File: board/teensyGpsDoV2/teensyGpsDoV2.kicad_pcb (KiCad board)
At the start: 2 copper layers, 12 parts, among them J1 Barrel_Jack, J2 NPPN042AFCN-RC, U1 Teensy4.0, U2 LT1086-5.0, U3 DAC8550IxDGK, X1 OSC5A2B02

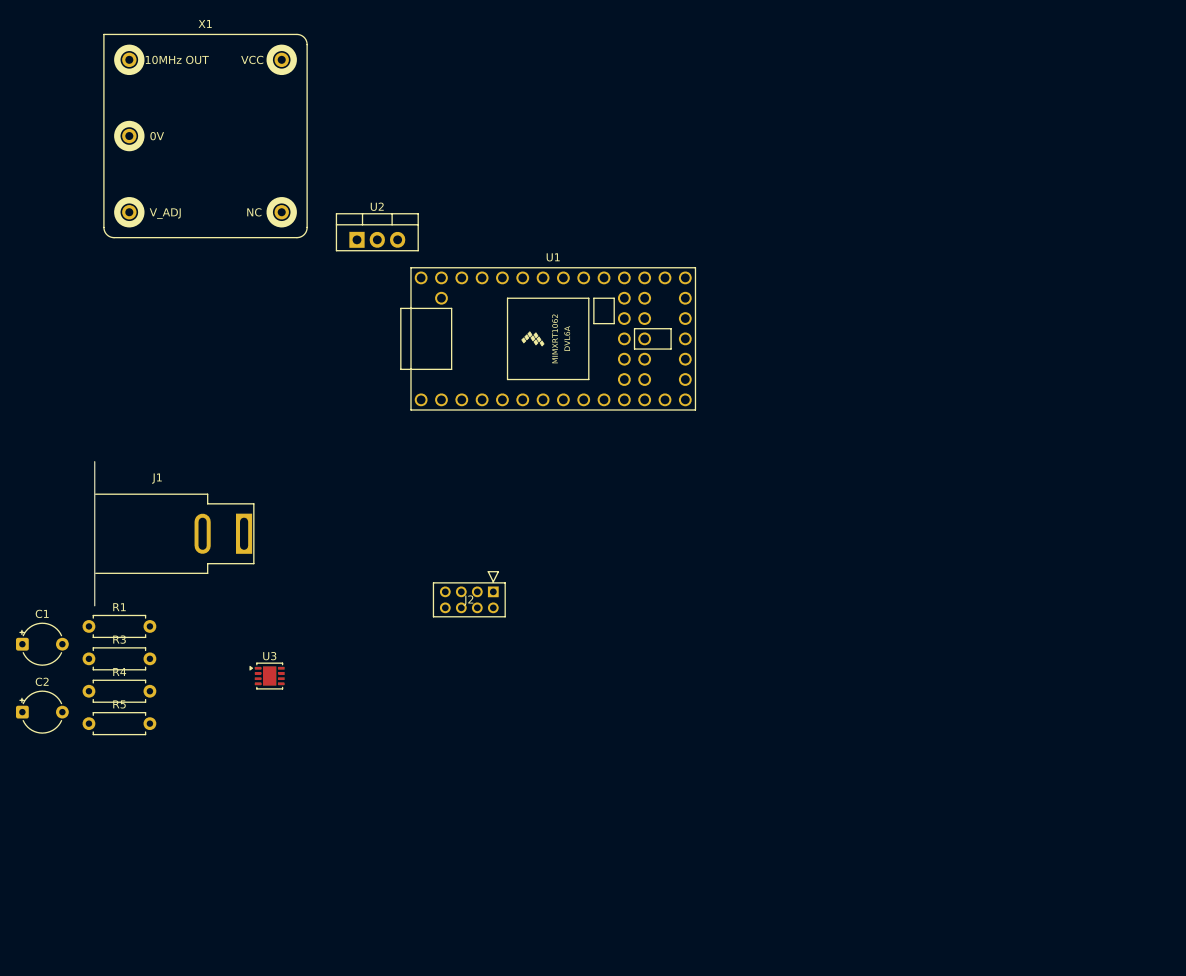
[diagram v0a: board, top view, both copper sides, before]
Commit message: layout wip
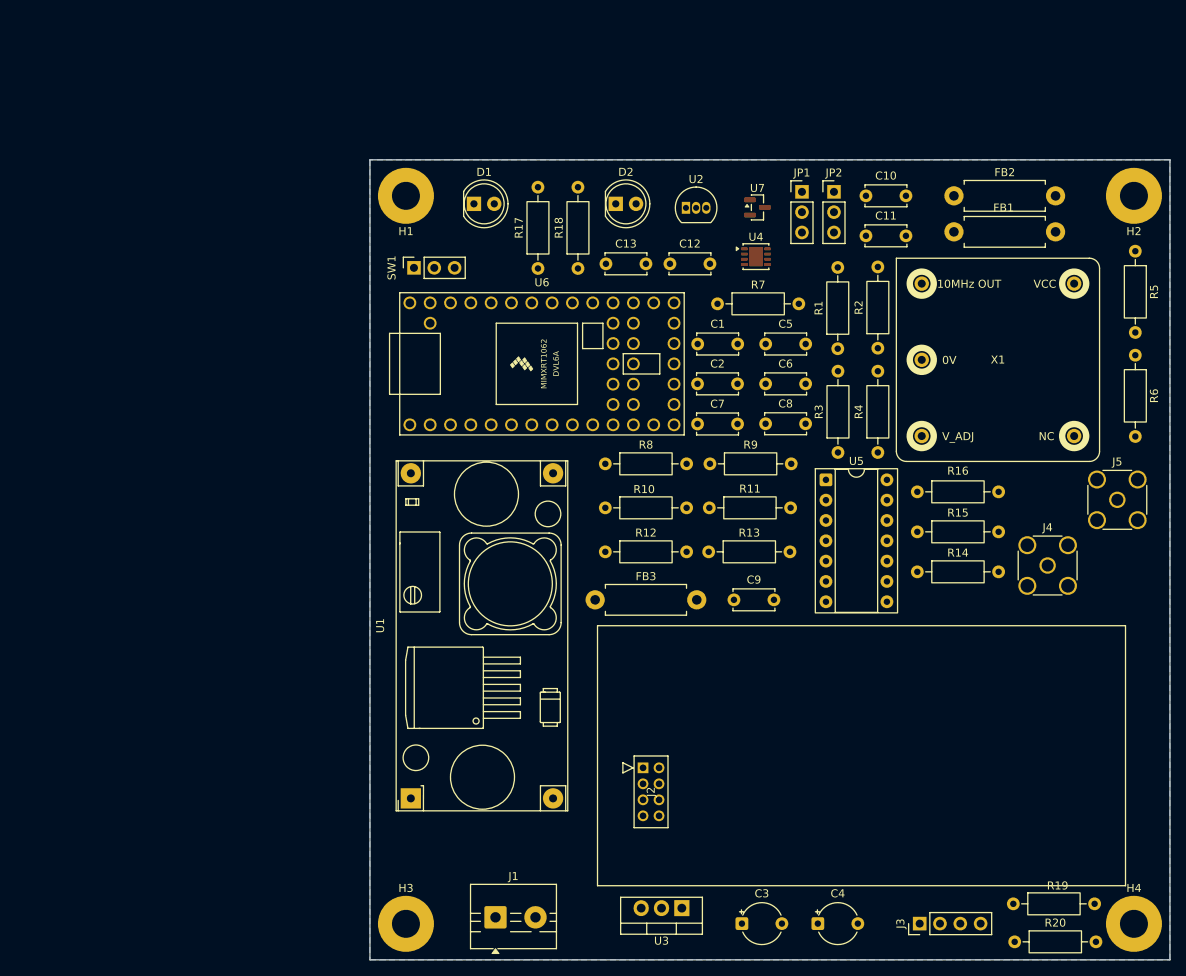
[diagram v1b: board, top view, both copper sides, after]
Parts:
- added C1: 1uF, Capacitor_THT:C_Disc_D5.0mm_W2.5mm_P5.00mm, F.Cu at (140.0, 69.0)
- added C10: 10uF, Capacitor_THT:C_Disc_D5.0mm_W2.5mm_P5.00mm, F.Cu at (161.1, 50.5)
- added C11: .1uF, Capacitor_THT:C_Disc_D5.0mm_W2.5mm_P5.00mm, F.Cu at (161.1, 55.5)
- added C12: 1uF, Capacitor_THT:C_Disc_D5.0mm_W2.5mm_P5.00mm, F.Cu at (136.6, 59.0)
- added C13: 1uF, Capacitor_THT:C_Disc_D5.0mm_W2.5mm_P5.00mm, F.Cu at (128.6, 59.0)
- added C2: 1uF, Capacitor_THT:C_Disc_D5.0mm_W2.5mm_P5.00mm, F.Cu at (140.0, 74.0)
- added C5: 10uF, Capacitor_THT:C_Disc_D5.0mm_W2.5mm_P5.00mm, F.Cu at (148.5, 69.0)
- added C6: .1uF, Capacitor_THT:C_Disc_D5.0mm_W2.5mm_P5.00mm, F.Cu at (148.5, 74.0)
- added C7: 10uF, Capacitor_THT:C_Disc_D5.0mm_W2.5mm_P5.00mm, F.Cu at (140.0, 79.0)
- added C8: 10uF, Capacitor_THT:C_Disc_D5.0mm_W2.5mm_P5.00mm, F.Cu at (148.5, 79.0)
- added C9: .1uF, Capacitor_THT:C_Disc_D5.0mm_W2.5mm_P5.00mm, F.Cu at (144.6, 101.0)
- added D1: PPS LED, LED_THT:LED_D5.0mm_Clear, F.Cu at (112.1, 51.5)
- added D2: Lock LED, LED_THT:LED_D5.0mm_Clear, F.Cu at (129.8, 51.5)
- added FB1: 133 @ 100 MHz, Resistor_THT:R_Axial_DIN0411_L9.9mm_D3.6mm_P12.70mm_Horizontal, F.Cu at (172.1, 55.0)
- added FB2: 133 @ 100 MHz, Resistor_THT:R_Axial_DIN0411_L9.9mm_D3.6mm_P12.70mm_Horizontal, F.Cu at (172.1, 50.5)
- added FB3: 133 @ 100 MHz, Resistor_THT:R_Axial_DIN0411_L9.9mm_D3.6mm_P12.70mm_Horizontal, F.Cu at (127.2, 101.0)
- added H1: MountingHole, MountingHole:MountingHole_3.5mm_Pad, F.Cu at (103.6, 50.5)
- added H2: MountingHole, MountingHole:MountingHole_3.5mm_Pad, F.Cu at (194.6, 50.5)
- added H3: MountingHole, MountingHole:MountingHole_3.5mm_Pad, F.Cu at (103.6, 141.5)
- added H4: MountingHole, MountingHole:MountingHole_3.5mm_Pad, F.Cu at (194.6, 141.5)
- added J3: LCD_Header, Connector_PinHeader_2.54mm:PinHeader_1x04_P2.54mm_Vertical, F.Cu at (167.8, 141.5)
- added J4: 10MHz Out, Connector_Coaxial:SMA_Wurth_60312002114503_Vertical, F.Cu at (183.8, 96.7)
- added J5: 1PPS Out, Connector_Coaxial:SMA_Wurth_60312002114503_Vertical, F.Cu at (192.5, 88.5)
- added JP1: OSC_VCTRL_SEL, Connector_PinHeader_2.54mm:PinHeader_1x03_P2.54mm_Vertical, F.Cu at (153.1, 50.0)
- added JP2: DAC_VREF_SEL, Connector_PinHeader_2.54mm:PinHeader_1x03_P2.54mm_Vertical, F.Cu at (157.1, 50.0)
- added R10: 33, Resistor_THT:R_Axial_DIN0207_L6.3mm_D2.5mm_P10.16mm_Horizontal, F.Cu at (128.5, 89.5)
- added R11: 33, Resistor_THT:R_Axial_DIN0207_L6.3mm_D2.5mm_P10.16mm_Horizontal, F.Cu at (141.5, 89.5)
- added R12: 33, Resistor_THT:R_Axial_DIN0207_L6.3mm_D2.5mm_P10.16mm_Horizontal, F.Cu at (128.5, 95.0)
- added R13: 100, Resistor_THT:R_Axial_DIN0207_L6.3mm_D2.5mm_P10.16mm_Horizontal, F.Cu at (141.4, 95.0)
- added R14: 100, Resistor_THT:R_Axial_DIN0207_L6.3mm_D2.5mm_P10.16mm_Horizontal, F.Cu at (167.5, 97.5)
- added R15: 100, Resistor_THT:R_Axial_DIN0207_L6.3mm_D2.5mm_P10.16mm_Horizontal, F.Cu at (167.5, 92.5)
- added R16: 4.7k, Resistor_THT:R_Axial_DIN0207_L6.3mm_D2.5mm_P10.16mm_Horizontal, F.Cu at (167.5, 87.5)
- added R17: 220, Resistor_THT:R_Axial_DIN0207_L6.3mm_D2.5mm_P10.16mm_Horizontal, F.Cu at (120.1, 59.6)
- added R18: 220, Resistor_THT:R_Axial_DIN0207_L6.3mm_D2.5mm_P10.16mm_Horizontal, F.Cu at (125.1, 59.6)
- added R19: 4.7k, Resistor_THT:R_Axial_DIN0207_L6.3mm_D2.5mm_P10.16mm_Horizontal, F.Cu at (179.5, 139.0)
- added R2: 100, Resistor_THT:R_Axial_DIN0207_L6.3mm_D2.5mm_P10.16mm_Horizontal, F.Cu at (162.6, 69.5)
- added R20: 4.7k, Resistor_THT:R_Axial_DIN0207_L6.3mm_D2.5mm_P10.16mm_Horizontal, F.Cu at (179.7, 143.8)
- added R6: 33, Resistor_THT:R_Axial_DIN0207_L6.3mm_D2.5mm_P10.16mm_Horizontal, F.Cu at (194.8, 70.4)
- added R7: 100, Resistor_THT:R_Axial_DIN0207_L6.3mm_D2.5mm_P10.16mm_Horizontal, F.Cu at (142.5, 64.0)
- added R8: 20k, Resistor_THT:R_Axial_DIN0207_L6.3mm_D2.5mm_P10.16mm_Horizontal, F.Cu at (128.5, 84.0)
- added R9: 20k, Resistor_THT:R_Axial_DIN0207_L6.3mm_D2.5mm_P10.16mm_Horizontal, F.Cu at (141.6, 84.0)
- added SW1: SW_SPDT, Connector_PinSocket_2.54mm:PinSocket_1x03_P2.54mm_Vertical, F.Cu at (104.6, 59.5)
- added U1: LM2596_Module, LM2596_Module:YAAJ_DCDC_StepDown_LM2596, F.Cu at (104.2, 125.8)
- added U2: MCP1703, Package_TO_SOT_THT:TO-92_Inline, F.Cu at (138.6, 52.0)
- added U5: 74HC14, Package_DIP:DIP-14_W7.62mm_Socket, F.Cu at (156.1, 86.0)
- added U7: REF3333, Package_TO_SOT_SMD:SOT-23, F.Cu at (147.5, 52.0)
- J1: value Barrel_Jack -> Screw_Terminal_01x02; footprint Connector_BarrelJack:BarrelJack_SwitchcraftConxall_RAPC10U_Horizontal -> TerminalBlock:TerminalBlock_MaiXu_MX126-5.0-02P_1x02_P5.00mm
- J2: value NPPN042AFCN-RC -> GPS Connector
- R1: value 330 -> 100; footprint Resistor_THT:R_Axial_DIN0207_L6.3mm_D2.5mm_P7.62mm_Horizontal -> Resistor_THT:R_Axial_DIN0207_L6.3mm_D2.5mm_P10.16mm_Horizontal
- R3: footprint Resistor_THT:R_Axial_DIN0207_L6.3mm_D2.5mm_P7.62mm_Horizontal -> Resistor_THT:R_Axial_DIN0207_L6.3mm_D2.5mm_P10.16mm_Horizontal
- R4: value 100 -> 330; footprint Resistor_THT:R_Axial_DIN0207_L6.3mm_D2.5mm_P7.62mm_Horizontal -> Resistor_THT:R_Axial_DIN0207_L6.3mm_D2.5mm_P10.16mm_Horizontal
- R5: value 100 -> 680; footprint Resistor_THT:R_Axial_DIN0207_L6.3mm_D2.5mm_P7.62mm_Horizontal -> Resistor_THT:R_Axial_DIN0207_L6.3mm_D2.5mm_P10.16mm_Horizontal
- U4: renamed from U3; value DAC8550IxDGK -> DAC8550
- moved R5 143.5 mm to (194.8, 57.4), turned to -90 degrees
- moved R4 103.0 mm to (162.6, 82.6), turned to 90 degrees
- moved X1 102.9 mm to (177.6, 71.0)
- moved C4 102.9 mm to (155.1, 141.5)
- moved R1 99.8 mm to (157.6, 69.6), turned to 90 degrees
- moved R3 97.1 mm to (157.6, 82.6), turned to 90 degrees
- moved C3 96.5 mm to (145.6, 141.5)
- moved U3 92.9 mm to (138.1, 139.5), turned to 180 degrees
- moved U4 80.3 mm to (147.3, 58.1)
- moved J1 57.3 mm to (114.8, 140.7)
- moved J2 28.9 mm to (133.2, 122.0), turned to 90 degrees
- moved U6 3.42 mm to (120.6, 71.5)
- renumbered C1 to C3, C2 to C4, U2 to U3, U1 to U6
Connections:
- net Net-(U1-20_A6_TX5_LRCLK1) renamed MCU_TO_GPS_UART
- net Net-(U1-21_A7_RX5_BCLK1) renamed GPS_TO_MCU_UART
- C3 pad 1: Net-(U2-VI) -> Net-(J1-Pin_2)
- C4 pad 1: +5V -> +5VD
- J1 pad 1: Net-(U2-VI) -> GND
- J1 pad 2: GND -> Net-(J1-Pin_2)
- J2 pad 6: pps -> Net-(J2-Pad6)
- R1 pad 1: 10 MHz -> DAC_DAT_CLK
- R1 pad 2: Net-(R1-Pad2) -> Net-(U4-SCLK)
- R3 pad 1: Net-(U1-13_SCK_CRX1_LED) -> DAC_CS
- R3 pad 2: Net-(U3-SCLK) -> Net-(U4-~{SYNC})
- R4 pad 1: Net-(U1-11_MOSI_CTX1) -> Net-(X1-OUT)
- R4 pad 2: Net-(U3-D_{IN}) -> Net-(R4-Pad2)
- R5 pad 1: Net-(U1-10_CS_MQSR) -> Net-(R4-Pad2)
- R5 pad 2: Net-(U3-~{SYNC}) -> GND
- U3 pad 2: +5V -> +5VD
- U3 pad 3: Net-(U2-VI) -> Net-(J1-Pin_2)
- U4 pad 1: +3.3V -> Net-(U4-V_{DD})
- U4 pad 2: unconnected-(U3-V_{REF}-Pad2) -> Net-(JP2-C)
- U4 pad 3: Net-(U3-V_{FB}) -> DAC OSC VCTRL
- U4 pad 4: Net-(U3-V_{FB}) -> DAC OSC VCTRL
- U4 pad 5: Net-(U3-~{SYNC}) -> Net-(U4-~{SYNC})
- U4 pad 6: Net-(U3-SCLK) -> Net-(U4-SCLK)
- U4 pad 7: Net-(U3-D_{IN}) -> Net-(U4-D_{IN})
- U6 pad 12: Net-(U1-10_CS_MQSR) -> DAC_CS
- U6 pad 13: Net-(U1-11_MOSI_CTX1) -> DAC_DAT
- U6 pad 20: Net-(U1-13_SCK_CRX1_LED) -> DAC_DAT_CLK
- U6 pad 21: unconnected-(U1-14_A0_TX3_SPDIF_OUT-Pad21) -> PPS_LED
- U6 pad 22: unconnected-(U1-15_A1_RX3_SPDIF_IN-Pad22) -> LOCK_LED
- U6 pad 23: unconnected-(U1-16_A2_RX4_SCL1-Pad23) -> LCD_SCL
- U6 pad 24: unconnected-(U1-17_A3_TX4_SDA1-Pad24) -> LCD_SDA
- U6 pad 25: pps -> 1PPS
- U6 pad 26: 10 MHz -> 10MHz_MCU
- U6 pad 33: /5V Teensy -> Net-(SW1-B)
- U6 pad 5: unconnected-(U1-3_LRCLK2-Pad5) -> PWM_OSC_TUNE
- X1 pad 1: 10 MHz -> Net-(X1-OUT)
- X1 pad 3: Net-(U3-V_{FB}) -> Net-(X1-VCTRL)
- X1 pad 5: +5V -> Net-(X1-VCC)
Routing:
- added copper zone on B.Cu, net GND
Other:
- board outline added: 100 x 100 mm
